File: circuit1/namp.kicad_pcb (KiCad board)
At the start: 2 copper layers, 159 x 111.5 mm, 97 parts, among them J1 Screw_Terminal_01x08, J2 Screw_Terminal_01x04, J3 Screw_Terminal_01x04, J4 Conn_01x08_Female, U1 NRF52840-DONGLE, U2 MCP6004, U3 MCP6004, U4 MCP1501-33xSN, U5 MCP3564, U6 MCP1754S-5002xCB, U7 MCP1754S-5002xCB, U8 MCP1754S-3302xCB

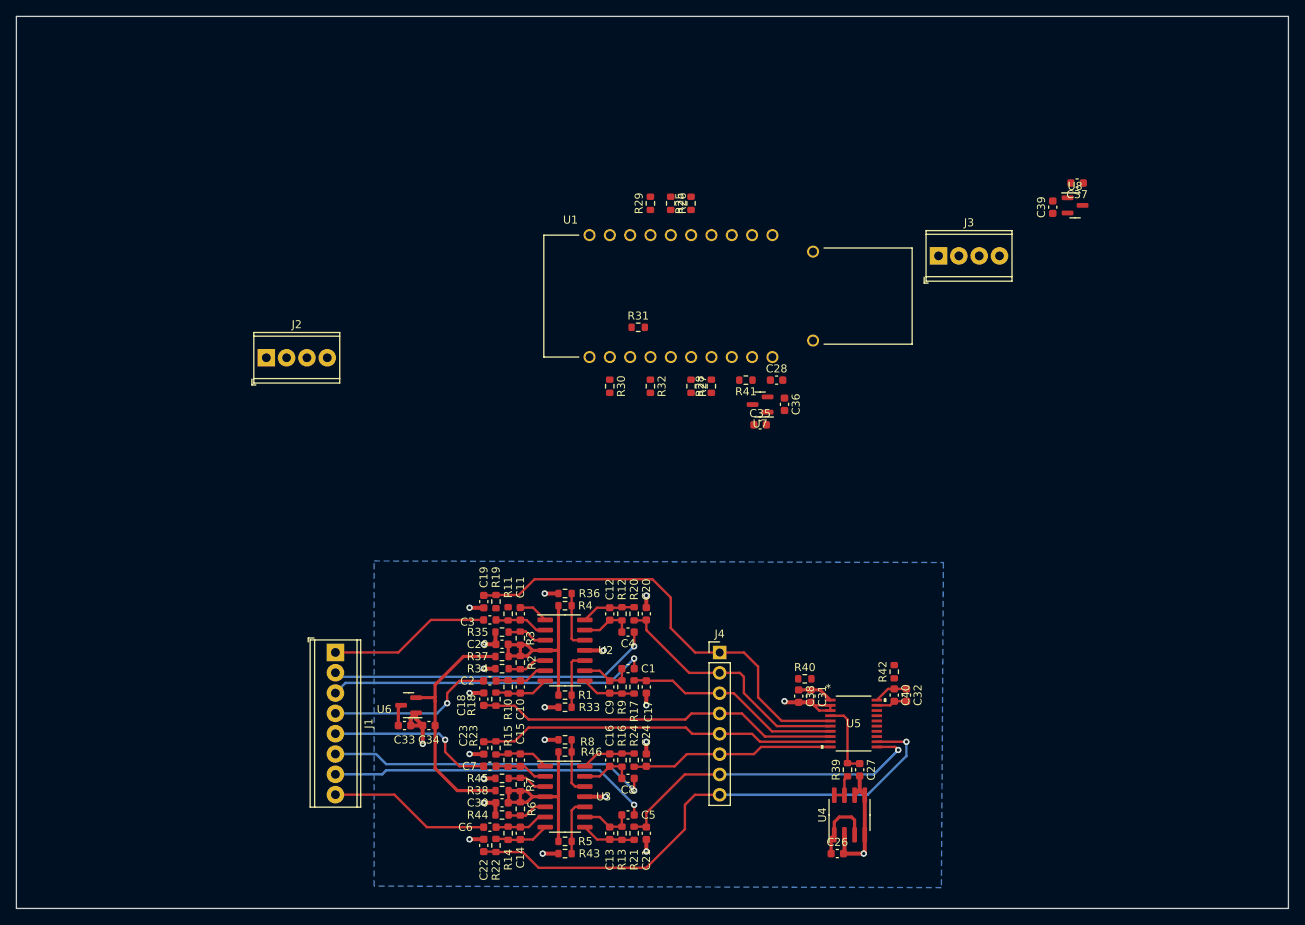
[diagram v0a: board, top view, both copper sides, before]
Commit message: update
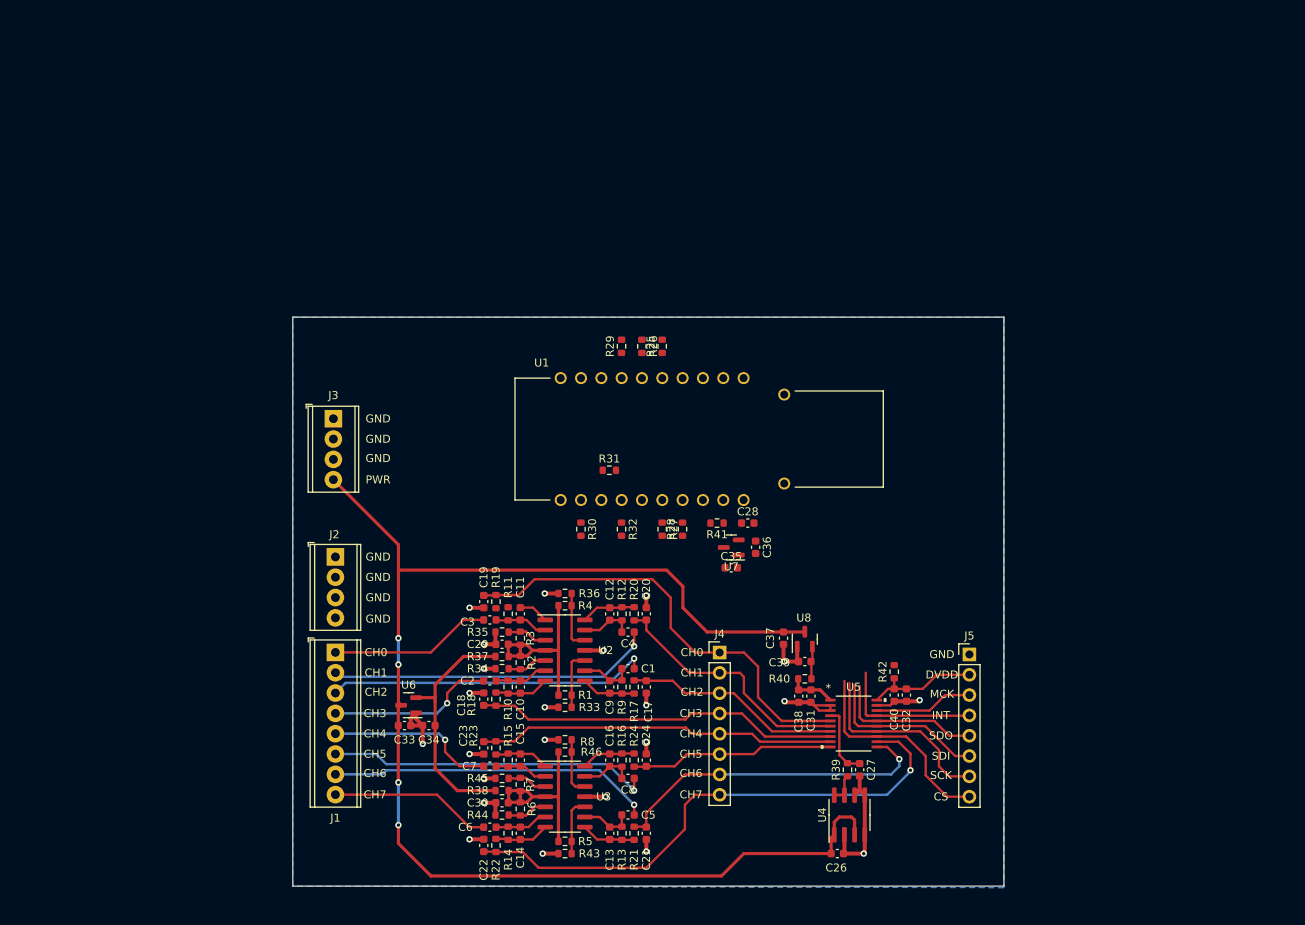
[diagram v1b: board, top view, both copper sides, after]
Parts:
- added J5: Conn_01x08_Male, Connector_PinHeader_2.54mm:PinHeader_1x08_P2.54mm_Vertical, F.Cu at (181.1, 128.5)
- moved J3 78.3 mm to (101.6, 99.1), turned to -90 degrees
- moved C37 67.7 mm to (157.9, 126.5), turned to -90 degrees
- moved C39 64.7 mm to (160.5, 129.4), turned to 180 degrees
- moved U8 63.9 mm to (160.5, 126.6), turned to 90 degrees
- moved J2 26.3 mm to (101.9, 116.3), turned to -90 degrees
- moved R26 18.2 mm to (140.2, 90.0)
- moved R30 18.2 mm to (132.5, 112.9)
- moved R41 18.2 mm to (149.6, 112.1)
- moved C28 18.2 mm to (153.4, 112.1)
- moved R25 18.2 mm to (142.7, 90.0)
- moved R27 18.2 mm to (142.7, 112.9)
- moved R28 18.2 mm to (145.2, 112.9)
- moved R29 18.2 mm to (137.6, 90.0)
- moved R31 18.2 mm to (136.1, 105.5)
- moved R32 18.2 mm to (137.6, 112.9)
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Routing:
- net PWR_MAX16V: track 11.6 -> 170.6 mm, vias 0 -> 4
- net ADC_CS: track 0.00 -> 26.8 mm
- net ADC_SCK: track 0.00 -> 24.4 mm
- net ADC_SDI: track 0.00 -> 20.8 mm
- net ADC_SDO: track 0.00 -> 18.6 mm
- net ADC_INT: track 0.00 -> 18.2 mm
- net ADC_MCK: track 0.00 -> 12.4 mm
- net ADC_DVDD: track 4.28 -> 14.2 mm
- net GND: track 71.1 -> 78.7 mm, vias 21 -> 23
- net Net-(C39-Pad1): track 0.00 -> 4.11 mm
- net ADC_AVDD: track 4.49 -> 5.90 mm
- net /ADC_CH7: track 66.7 -> 68.0 mm
- net /ADC_CH6: track 40.9 -> 41.7 mm
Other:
- board size 159 x 111.5 mm -> 88.9 x 71.1 mm
- board text added: "CH0"
- board text added: "CH1"
- board text added: "CH2"
- board text added: "CH3"
- board text added: "CH4"
- board text added: "CH5"
- board text added: "CH6"
- board text added: "CH7"
- board text added: "CS"
- board text added: "DVDD"
- board text added: "GND"
- board text added: "INT"
- board text added: "MCK"
- board text added: "PWR"
- board text added: "SCK"
- board text added: "SDI"
- board text added: "SDO"
